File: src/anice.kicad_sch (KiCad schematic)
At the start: 7 parts, among them J1 Conn_02x20_Counter_Clockwise, U1 ECP5U_12_CABGA256

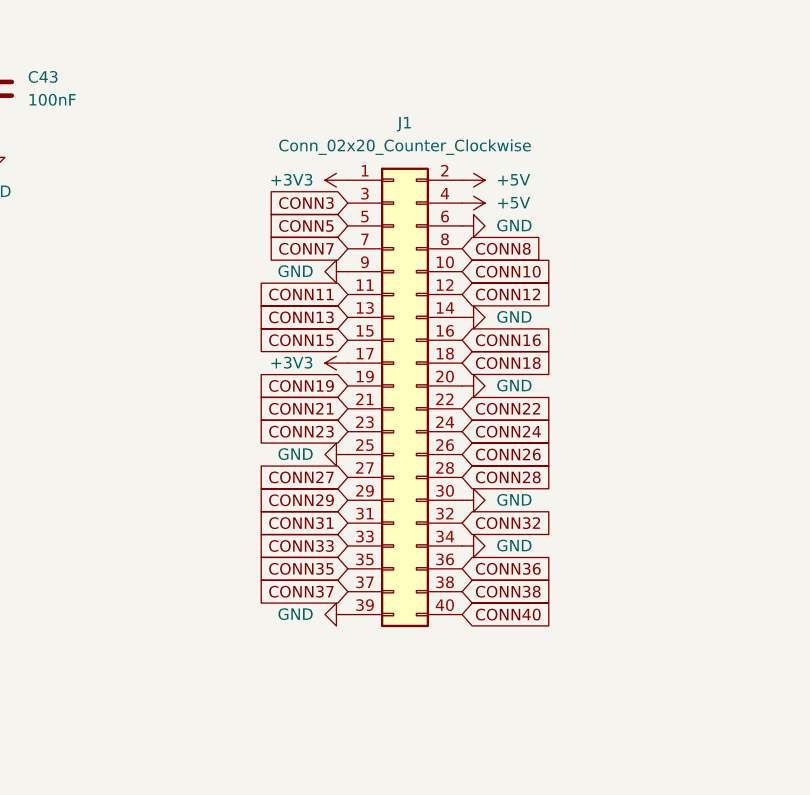
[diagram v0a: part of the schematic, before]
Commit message: Rev 2
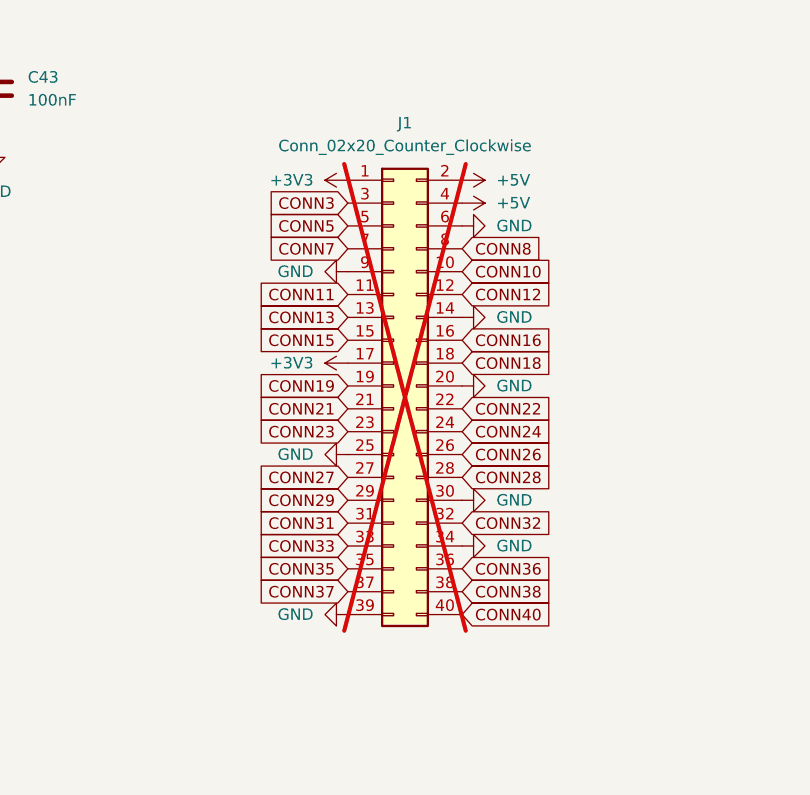
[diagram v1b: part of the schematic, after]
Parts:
- C43: LCSC Part (none) -> C1525
- J1: now not fitted
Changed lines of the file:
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@@
 			)
 		)
-		(property "LCSC Part" ""
+		(property "LCSC Part" "C1525"
 			(at 151.13 27.94 0)
 			(effects
@@
 		(in_bom yes)
 		(on_board yes)
-		(dnp no)
+		(dnp yes)
 		(fields_autoplaced yes)
 		(property "Reference" "J1"

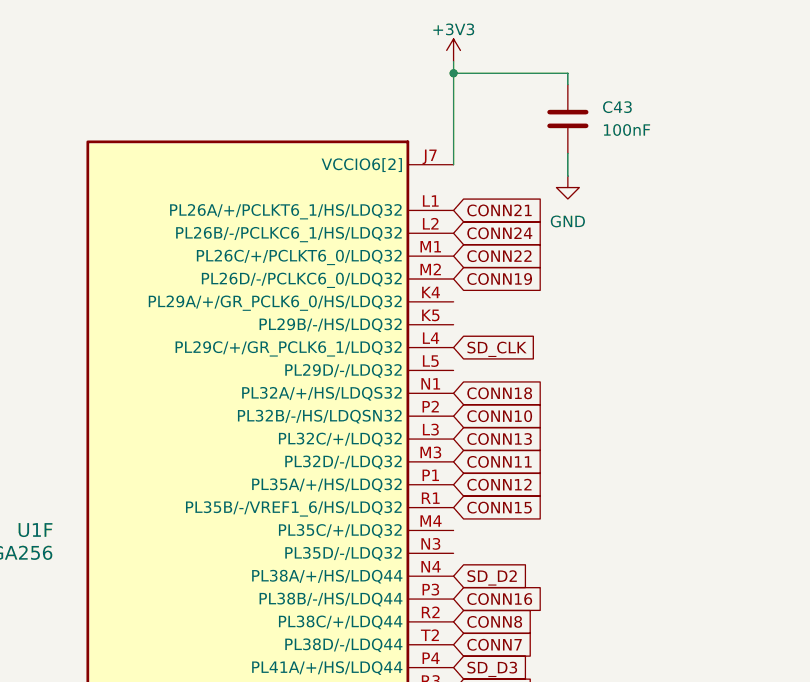
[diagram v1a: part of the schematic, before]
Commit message: Tidy project
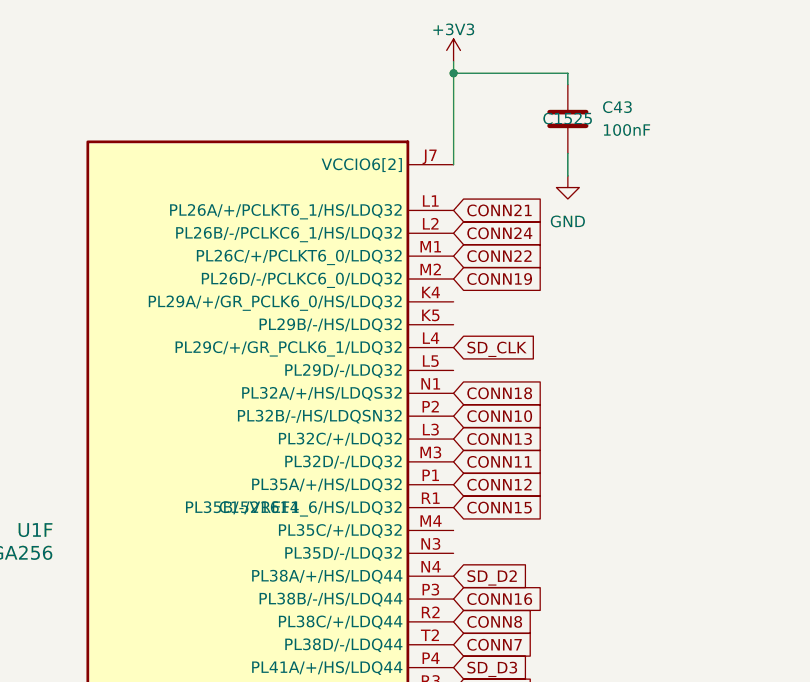
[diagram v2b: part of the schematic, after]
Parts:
- C43: JLCPCB Part # (none) -> C1525; LCSC Part C1525 -> (none)
- U1: JLCPCB Part # (none) -> C1521614; LCSC Part C1521614 -> (none)
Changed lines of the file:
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@@
 			)
 		)
-		(property "LCSC Part" "C1525"
+		(property "JLCPCB Part #" "C1525"
 			(at 151.13 27.94 0)
 			(effects
@@
 					(size 1.27 1.27)
 				)
-				(hide yes)
 			)
 		)
@@
 			)
 		)
-		(property "LCSC Part" ""
-			(at 252.73 147.32 0)
-			(effects
-				(font
-					(size 1.27 1.27)
-				)
-				(hide yes)
-			)
-		)
 		(instances
 			(project "anice"
@@
 		)
 		(property "Description" "Generic connector, double row, 02x20, odd/even pin numbering scheme (row 1 odd numbers, row 2 even numbers), script generated (kicad-library-utils/schlib/autogen/connector/)"
-			(at 195.58 60.96 0)
-			(effects
-				(font
-					(size 1.27 1.27)
-				)
-				(hide yes)
-			)
-		)
-		(property "LCSC Part" ""
 			(at 195.58 60.96 0)
 			(effects
@@
 			)
 		)
-		(property "LCSC Part" " C1521614"
+		(property "JLCPCB Part #" " C1521614"
 			(at 116.84 71.12 0)
 			(effects
@@
 					(size 1.27 1.27)
 				)
-				(hide yes)
-			)
-		)
+			)
+		)
